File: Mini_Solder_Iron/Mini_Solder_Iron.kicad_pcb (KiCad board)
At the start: 4 copper layers, 100 x 13 mm, 87 parts, among them CN1 YXT-BB10-24S-02, J1 USB_C_Receptacle_USB2.0, J2 Negative, J3 Positive, J4 Conn_01x04, J5 Conn_01x04, J6 Conn_01x04, J7 Com, Q1 AO4407A, Q2 MMBT3904, SW1 SW_Push, SW2 SW_Push, U1 STM32F103C8T6, U2 LIS2DS12, U3 SGM8557-1AXN5G/TR, U4 TMP36GRTZ, U5 CH340E, U6 MP9942, U7 CH224K, U8 LP5907MFX-3.3, U9 LP5907MFX-1.8, Y1 Crystal_GND3_Small

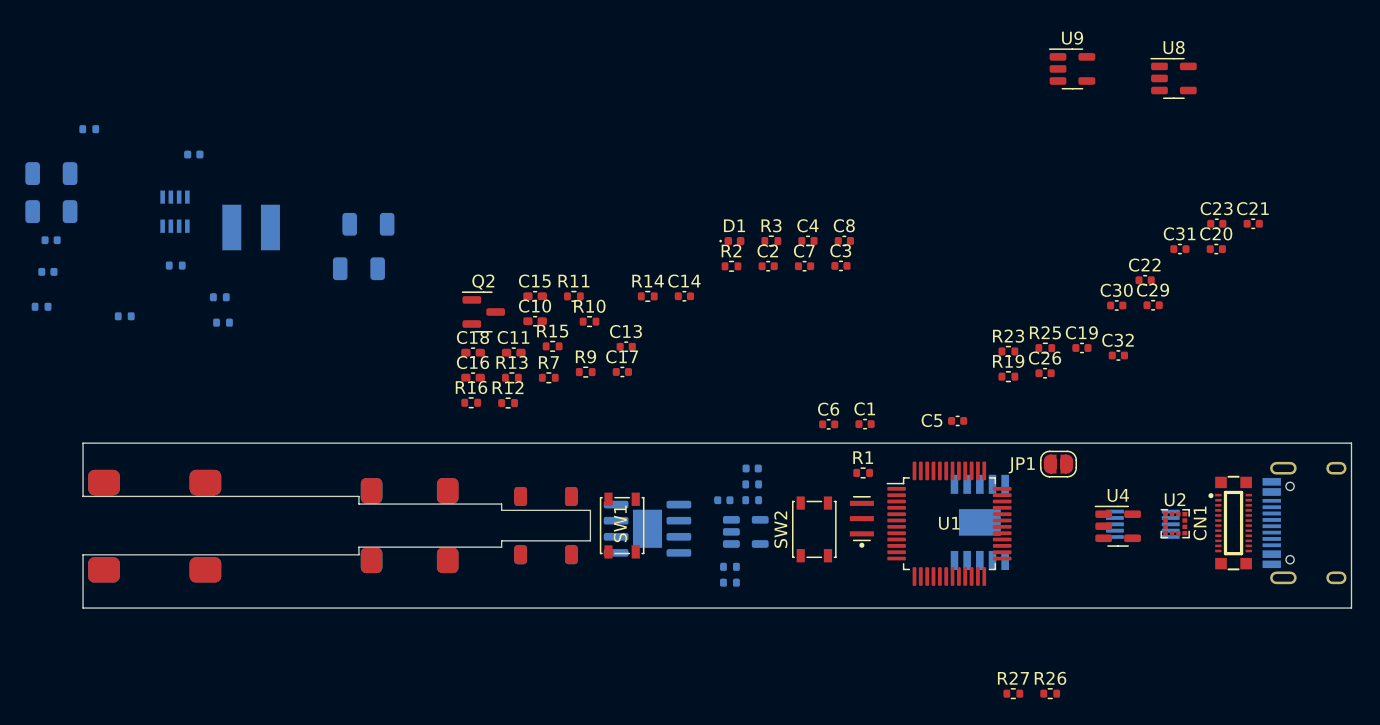
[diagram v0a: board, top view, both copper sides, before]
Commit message: update
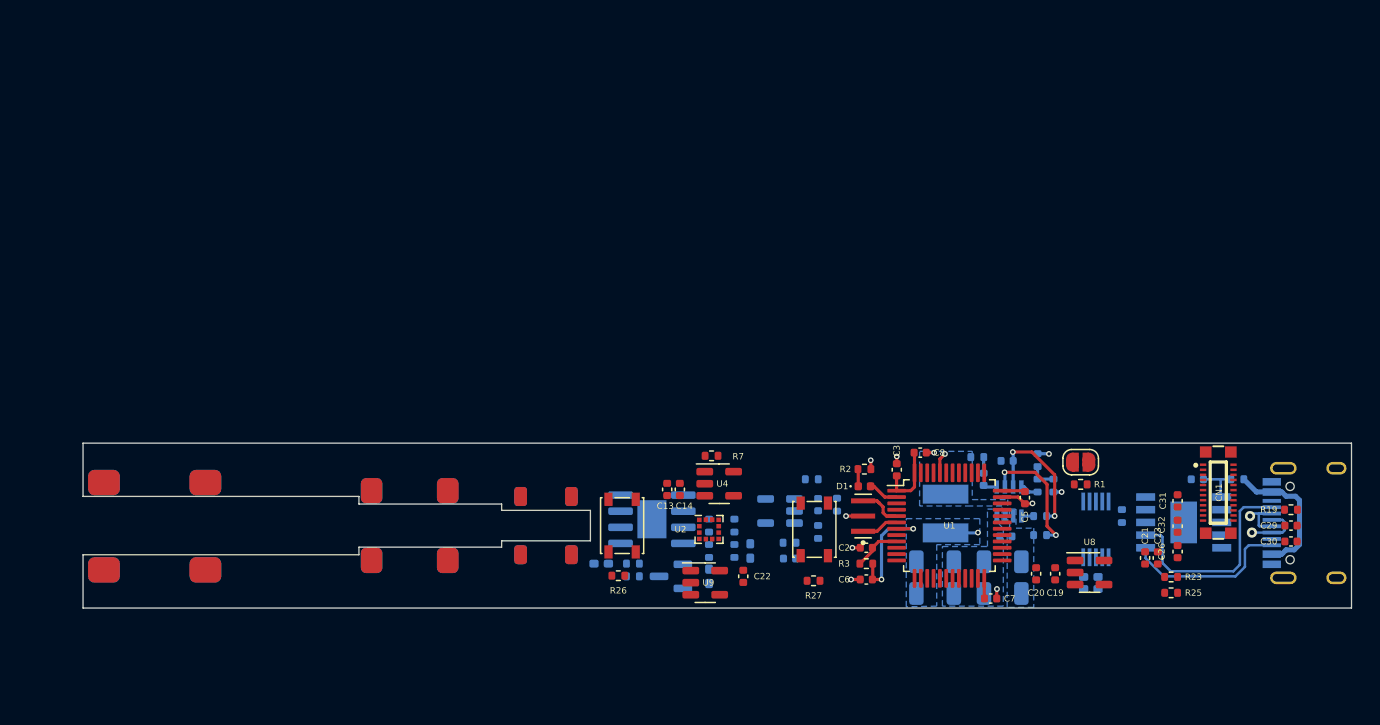
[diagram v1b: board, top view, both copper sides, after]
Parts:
- removed C1, C4: 30PF, Capacitor_SMD:C_0402_1005Metric
- C10, C11, C15, C16, C17, C18, Q2, R10, R11, R12, R13, R14, R15, R16, R9: moved to B.Cu
- moved C24 82.0 mm to (189.2, 97.8), turned to 0 degrees
- moved C25 79.9 mm to (189.2, 95.3), turned to 0 degrees
- moved R24 79.4 mm to (192.0, 87.2), turned to 90 degrees
- moved C27 78.8 mm to (189.5, 93.3), turned to 0 degrees
- moved C28 77.1 mm to (189.6, 87.3), turned to 0 degrees
- moved R21 74.6 mm to (187.2, 87.0)
- moved R20 73.2 mm to (192.0, 89.2), turned to 90 degrees
- moved R17 71.4 mm to (192.2, 93.2), turned to 0 degrees
- moved U6 69.6 mm to (189.8, 90.5)
- moved C33 67.3 mm to (187.8, 88.8), turned to -90 degrees
- moved R18 66.9 mm to (192.2, 91.7), turned to 0 degrees
- moved R22 66.7 mm to (193.2, 89.2), turned to -90 degrees
- moved L1 59.2 mm to (184.8, 91.5), turned to -90 degrees
- moved R13 57.7 mm to (207.8, 88.8), turned to 180 degrees
- moved C35 52.1 mm to (183.9, 97.8)
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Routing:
- net Net-(J1-PadA5): track 0.00 -> 16.9 mm
- net +5V: track 0.00 -> 14.2 mm, vias 0 -> 2
- net Net-(J1-PadB5): track 0.00 -> 13.2 mm
- net +3V3: track 0.00 -> 12.6 mm
- net VBUS: track 0.00 -> 11.1 mm
- net Net-(C28-Pad2): track 0.00 -> 10.7 mm, vias 0 -> 2
- net Net-(R17-Pad2): track 0.00 -> 9.94 mm, vias 0 -> 2
- net Net-(C6-Pad1): track 0.00 -> 9.47 mm, vias 0 -> 2
- net GND: track 0.00 -> 8.61 mm, vias 0 -> 9
- net USB_DM: track 0.00 -> 4.79 mm, vias 0 -> 1
- net USB_DP: track 0.00 -> 4.39 mm, vias 0 -> 1
- net Net-(C17-Pad1): track 0.00 -> 4.02 mm
- net HSE_IN: track 0.00 -> 3.41 mm
- net HSE_OUT: track 0.00 -> 2.93 mm
- net Net-(D1-Pad2): track 0.00 -> 2.40 mm
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- added copper zone on B.Cu, net +5V
- added copper zone on B.Cu, net GND
- added copper zone on B.Cu, net Net-(L1-Pad1)
- added copper zone on B.Cu, net VBUS

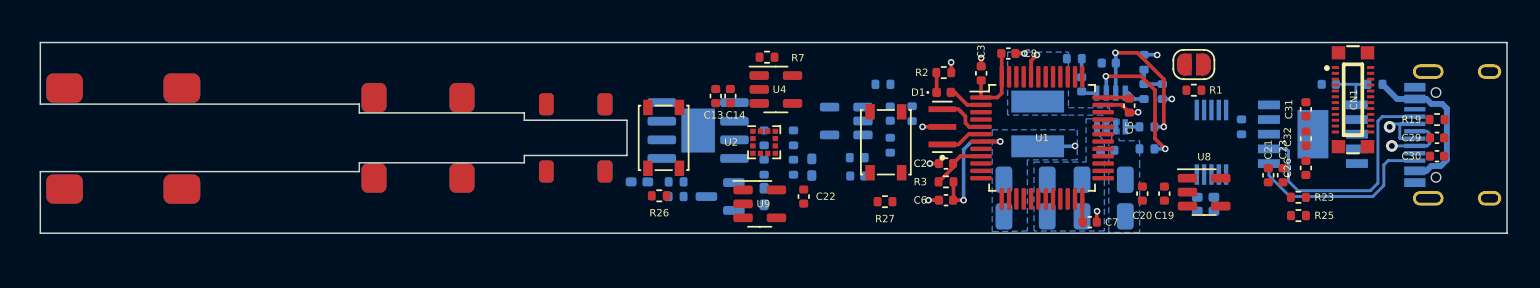
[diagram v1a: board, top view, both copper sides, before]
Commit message: PCB layout update
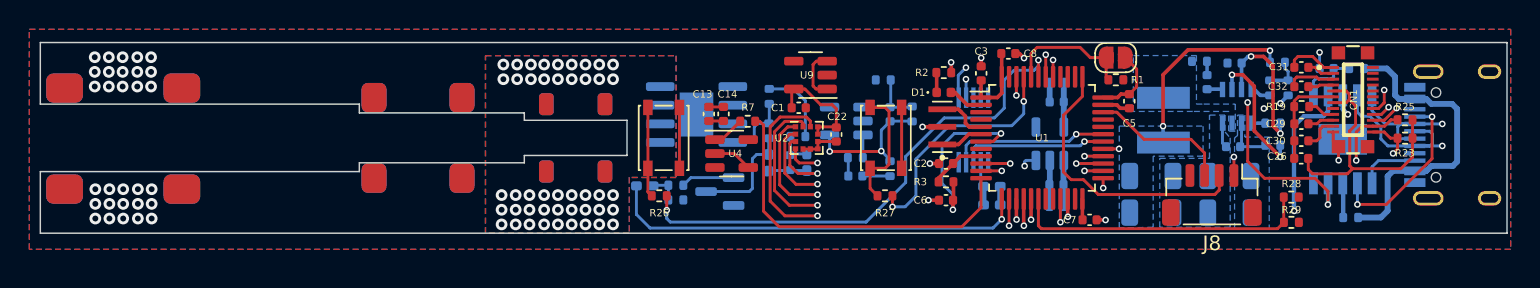
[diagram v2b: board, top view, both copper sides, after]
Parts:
- added C1: 1uF, Capacitor_SMD:C_0402_1005Metric, F.Cu at (168.5, 90.3)
- added J8: Conn_01x04, Connector_JST:JST_SH_BM04B-SRSS-TB_1x04-1MP_P1.00mm_Vertical, F.Cu at (196.6, 96.3)
- added R28: 1K, Resistor_SMD:R_0402_1005Metric, F.Cu at (202.0, 96.4)
- added R29: 1K, Resistor_SMD:R_0402_1005Metric, F.Cu at (202.1, 98.2)
- C19, C20, C21, C23, U8: moved to B.Cu
- moved C23 16.7 mm to (186.1, 88.6), turned to 0 degrees
- moved U5 16.3 mm to (180.4, 91.9)
- moved C21 15.3 mm to (186.1, 90.0), turned to 0 degrees
- moved C11 14.7 mm to (181.6, 95.7)
- moved C10 14.6 mm to (181.6, 97.0)
- moved U8 11.0 mm to (185.6, 92.8), turned to 90 degrees
- moved R25 9.77 mm to (209.8, 91.2), turned to 180 degrees
- moved R16 9.67 mm to (206.1, 97.8), turned to 0 degrees
- moved U9 9.44 mm to (169.3, 88.1), turned to 180 degrees
- moved C30 9.31 mm to (202.7, 92.6)
- moved C29 9.30 mm to (202.7, 91.4)
- moved R19 9.27 mm to (202.8, 90.3)
- moved R24 9.10 mm to (201.1, 87.2), turned to 180 degrees
- moved R17 8.58 mm to (200.8, 92.9)
- moved R18 8.58 mm to (200.8, 91.4)
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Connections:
- CN1 pad 17: CS -> DISPLAY_CS
- U1 pad 14: CS -> DISPLAY_CS
- U1 pad 15: SCK -> SCL
- U1 pad 16: MISO -> RESET
- U1 pad 17: MOSI -> SDA
- U1 pad 18: unconnected-(U1-Pad18) -> Voltage
- U1 pad 21: unconnected-(U1-Pad21) -> CFG2
- U1 pad 22: Button1 -> CFG3
- U1 pad 25: Button2 -> IMU_CS
- U1 pad 26: CFG1 -> IMU_SCK
- U1 pad 27: CFG2 -> IMU_SD0
- U1 pad 28: CFG3 -> IMU_SDA
- U1 pad 29: unconnected-(U1-Pad29) -> DCX
- U1 pad 32: INT1 -> USB_DP
- U1 pad 33: INT2 -> USB_DM
- U1 pad 41: unconnected-(U1-Pad41) -> INT2
- U1 pad 42: SCL -> INT1
- U1 pad 43: SDA -> Button1
- U1 pad 45: unconnected-(U1-Pad45) -> Button2
- U1 pad 46: unconnected-(U1-Pad46) -> CFG1
- U2 pad 1: SCK -> IMU_SCK
- U2 pad 2: CS -> IMU_CS
- U2 pad 3: SD0 -> IMU_SD0
- U2 pad 4: SDA -> IMU_SDA
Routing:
- net USB_DP: track 4.39 -> 56.7 mm, vias 1 -> 2
- net USB_DM: track 4.79 -> 50.2 mm, vias 1 -> 2
- net INT2: track 0.00 -> 43.7 mm, vias 0 -> 2
- net CFG3: track 0.00 -> 39.9 mm, vias 0 -> 2
- net IMU_SCK: track 0.00 -> 39.3 mm, vias 0 -> 2
- net INT1: track 0.00 -> 38.8 mm, vias 0 -> 2
- net Button1: track 0.00 -> 35.1 mm, vias 0 -> 2
- net DISPLAY_CS: track 0.00 -> 34.3 mm, vias 0 -> 2
- net RESET: track 0.00 -> 34.0 mm, vias 0 -> 2
- net +3V3: track 12.6 -> 45.3 mm, vias 0 -> 1
- net SCL: track 0.00 -> 32.1 mm, vias 0 -> 2
- net SDA: track 0.00 -> 31.8 mm, vias 0 -> 2
- net GND: track 8.61 -> 40.0 mm, vias 9 -> 11
- net CFG1: track 0.00 -> 30.2 mm, vias 0 -> 3
- net Tip_Control: track 0.00 -> 28.9 mm, vias 0 -> 1
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- added copper zone on B.Cu, net A
- added copper zone on F.Cu, net A
- added copper zone on F.Cu, net GND
- added copper zone on In1.Cu, net GND
- added copper zone on In2.Cu, net GND
